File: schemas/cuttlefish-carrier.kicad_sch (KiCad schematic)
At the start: 8 parts, among them J3 Motor_Socket, J4 Servo_Socket, J5 SBC_Socket, J6 Battery_Socket, SW1 SW_SPDT

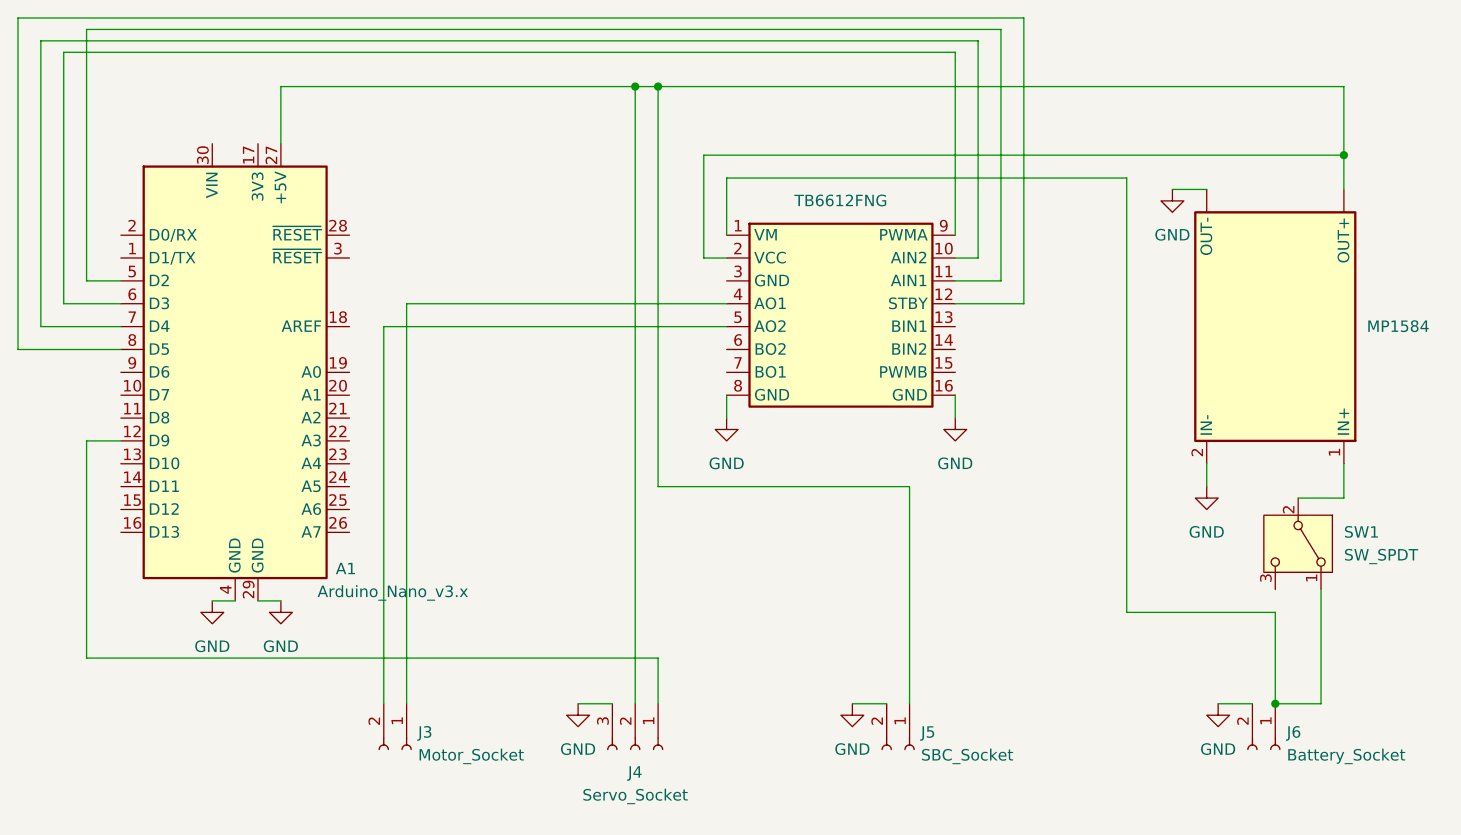
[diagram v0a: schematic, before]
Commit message: feat: update schemas
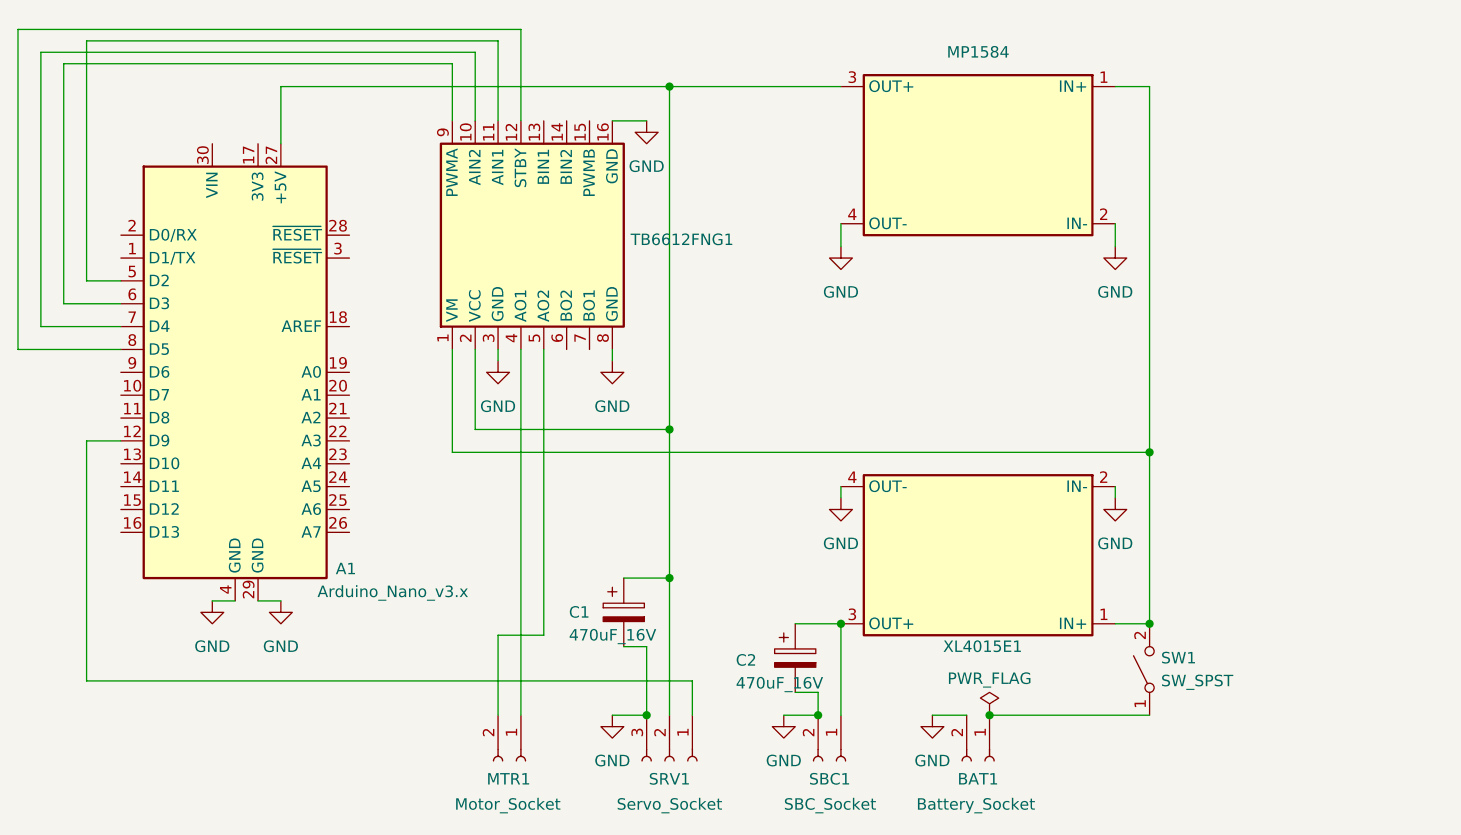
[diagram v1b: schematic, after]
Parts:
- removed SW1: SW_SPDT, Button_Switch_THT:SW_NKK_GW12LJP, symbol Switch:SW_SPDT
- removed TB6612FNG: (no value), Package_DFN_QFN:VQFN-16-1EP_3x3mm_P0.5mm_EP1.8x1.8mm, symbol Driver_Motor:TB6612FNG_breakout
- added C1, C2: 470uF_16V, Capacitor_THT:CP_Radial_D8.0mm_P3.50mm, symbol Device:C_Polarized
- added SW1: SW_SPST, TerminalBlock_Phoenix:TerminalBlock_Phoenix_MKDS-1,5-2_1x02_P5.00mm_Horizontal, symbol Switch:SW_SPST
- added TB6612FNG1: (no value), Connector_PinSocket_2.54mm:TB6612FNG_PinSocket, symbol Driver_Motor:TB6612FNG_breakout
- added XL4015E1: (no value), Connector_PinSocket_2.54mm:XL4015E_PinSocket, symbol Converter_DCDC:XL4015E
- A1: footprint Module:Arduino_Nano -> Module:Arduino_Nano_Socket
- BAT1: renamed from J6; footprint (none) -> TerminalBlock_Phoenix:TerminalBlock_Phoenix_MKDS-1,5-2_1x02_P5.00mm_Horizontal
- MP1584: footprint (none) -> Connector_PinSocket_2.54mm:MP1584_PinSocket
- MTR1: renamed from J3; footprint (none) -> TerminalBlock_Phoenix:TerminalBlock_Phoenix_MKDS-1,5-2_1x02_P5.00mm_Horizontal
- SBC1: renamed from J5; footprint (none) -> TerminalBlock_Phoenix:TerminalBlock_Phoenix_MKDS-1,5-2_1x02_P5.00mm_Horizontal
- SRV1: renamed from J4; footprint (none) -> Connector_PinHeader_2.54mm:PinHeader_1x03_P2.54mm_Horizontal
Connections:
- net GND: now also MP1584.4 (OUT-), C1.2, C2.2, TB6612FNG1.16 (GND), TB6612FNG1.3 (GND), TB6612FNG1.8 (GND), XL4015E1.2 (IN-), XL4015E1.4 (OUT-); no longer MP1584. (OUT-)
- net at BAT1.1 (Pin_1): now also SW1.1 (A)
- net at MP1584.1 (IN+): now also SW1.2 (B), TB6612FNG1.1 (VM), XL4015E1.1 (IN+)
- net at A1.27 (+5V), SRV1.2 (Pin_2): now also MP1584.3 (OUT+), C1.1, TB6612FNG1.2 (VCC); no longer MP1584. (OUT-), SBC1.1 (Pin_1)
- net at MTR1.1 (Pin_1): now also TB6612FNG1.4 (AO1)
- net at MTR1.2 (Pin_2): now also TB6612FNG1.5 (AO2)
- net at A1.5 (D2): now also TB6612FNG1.11 (AIN1)
- net at A1.6 (D3): now also TB6612FNG1.9 (PWMA)
- net at A1.7 (D4): now also TB6612FNG1.10 (AIN2)
- net at A1.8 (D5): now also TB6612FNG1.12 (STBY)
- new net: C2.1, SBC1.1 (Pin_1), XL4015E1.3 (OUT+)
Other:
- moved on the sheet: BAT1, MTR1, SBC1, SRV1
